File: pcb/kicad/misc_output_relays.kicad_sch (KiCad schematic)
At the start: 16 parts, among them J5 Screw_Terminal_01x03, J6 Screw_Terminal_01x03, K1 5v Relay, K2 5v Relay, Q1 MMBT3904-TP, Q2 MMBT3904-TP

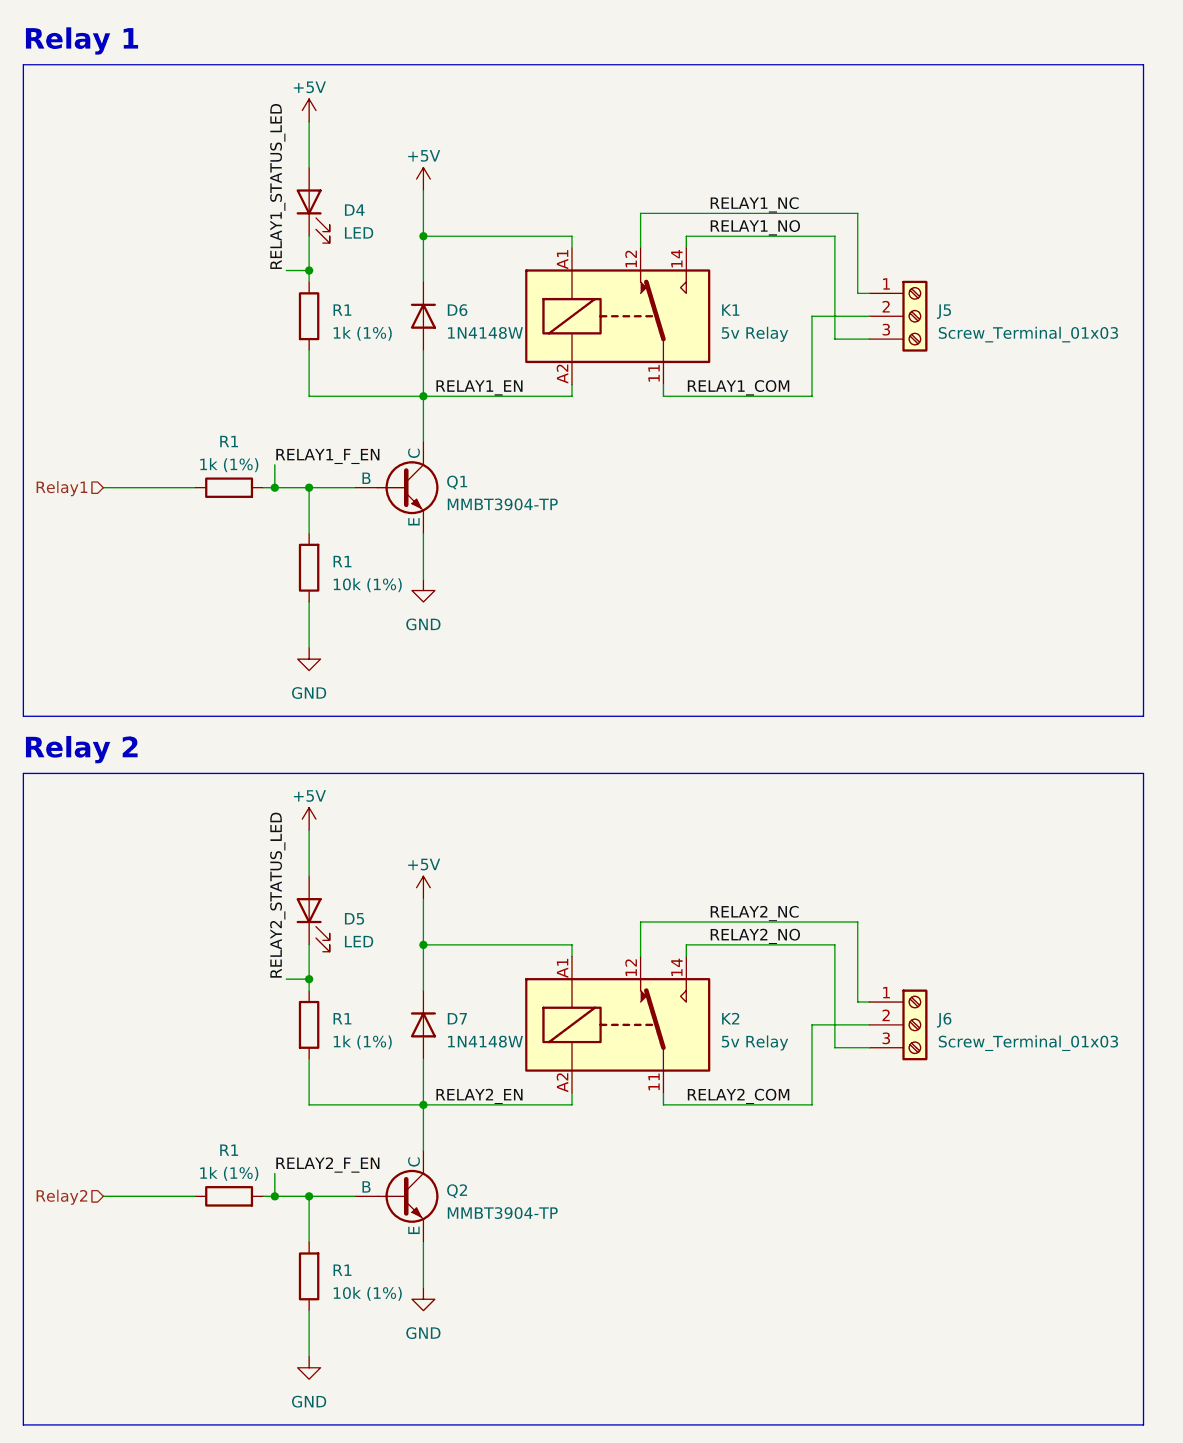
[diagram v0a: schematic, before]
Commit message: rev3-update
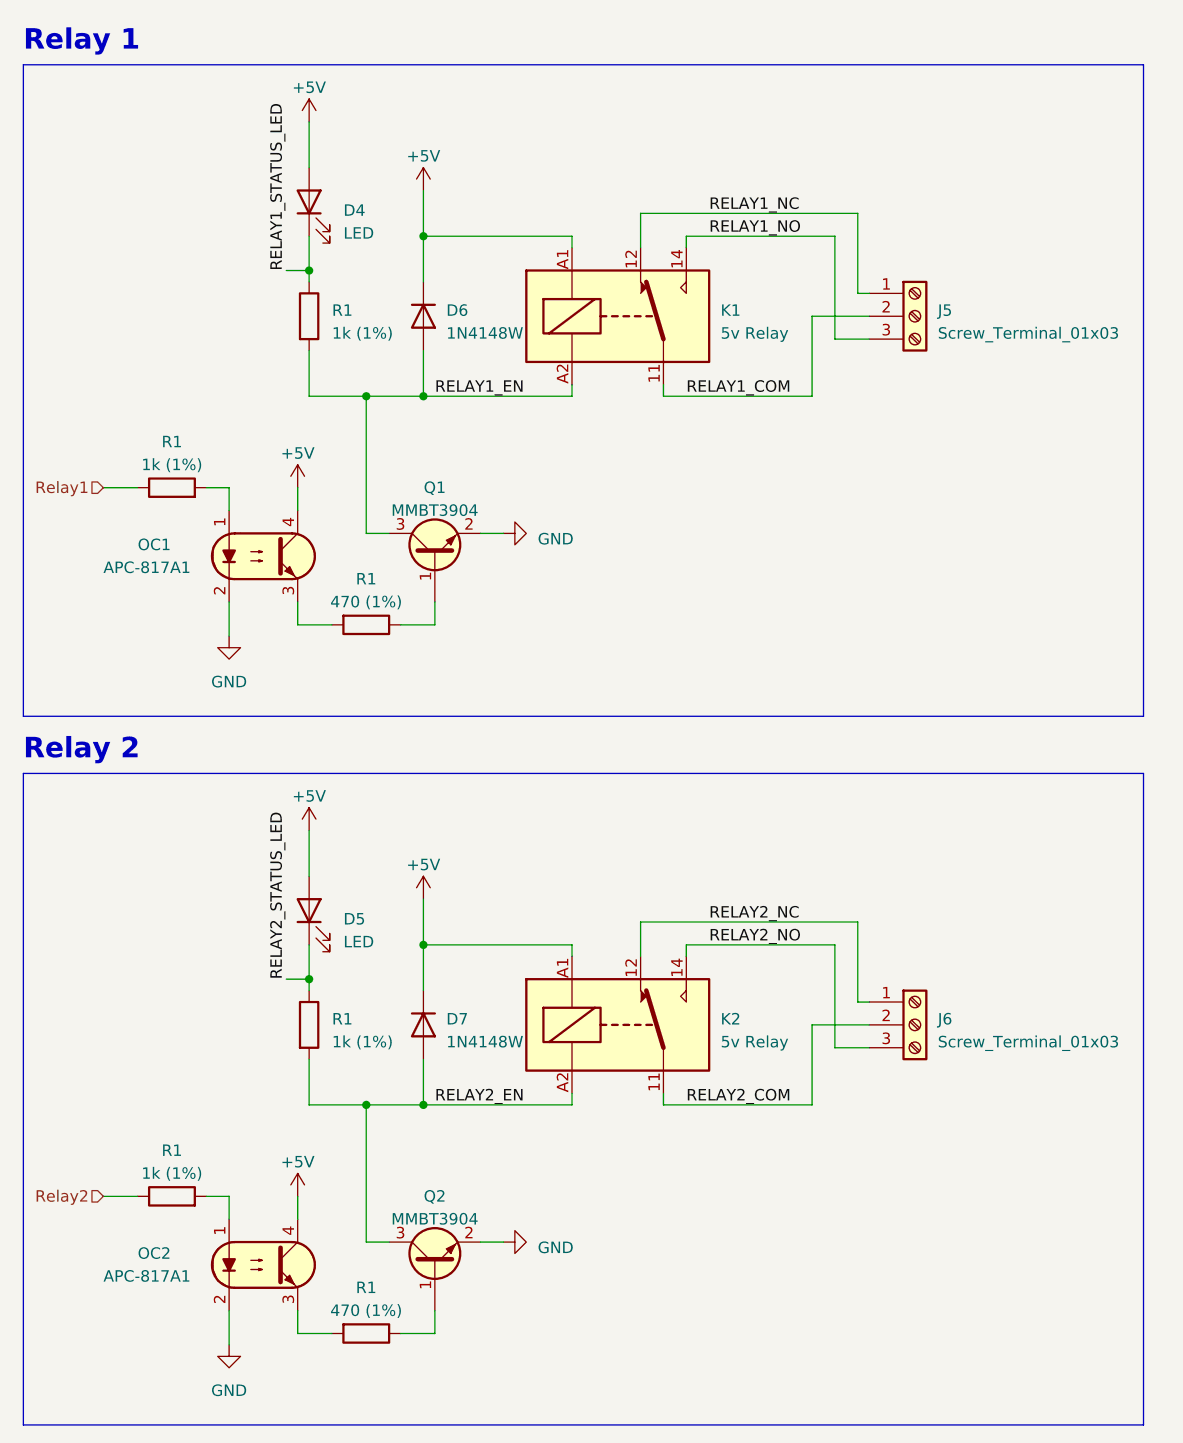
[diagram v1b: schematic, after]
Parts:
- removed Q1, Q2: MMBT3904-TP, Package_TO_SOT_SMD:SOT-23, symbol Simulation_SPICE:NPN
- removed R1: 10k (1%), PCM_Resistor_SMD_AKL:R_0603_1608Metric, symbol Device:R
- removed R1: 1k (1%), PCM_Resistor_SMD_AKL:R_0603_1608Metric, symbol Device:R
- added OC1, OC2: APC-817A1, LTV-816S:SMD4-2.54-4.6X6.5MM, symbol PCM_Optocoupler_AKL:Optocoupler_Generic
- added Q1, Q2: MMBT3904, Package_TO_SOT_SMD_AKL:SOT-23, symbol PCM_Transistor_BJT_AKL:MMBT3904
- added R1: 470 (1%), PCM_Resistor_SMD_AKL:R_0603_1608Metric, symbol Device:R
- added R1: 1k (1%), PCM_Resistor_SMD_AKL:R_0603_1608Metric, symbol Device:R
- R1: value 10k (1%) -> 470 (1%)
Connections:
- net +5V: now also OC1.4, OC2.4
- net GND: now also OC1.2, OC2.2, Q1.2 (E), Q2.2 (E); no longer R1.1
- net RELAY1_EN: now also Q1.3 (C)
- net RELAY2_EN: now also Q2.3 (C)
- net Relay2: now also R1.1
- net RELAY1_F_EN: no longer names the net of R1.2
- net RELAY1_F_EN: now also OC1.1; no longer R1.2
- new net: Q2.1 (B), R1.1
- new net: OC2.3, R1.2
- new net: Q1.1 (B), R1.1
- new net: OC1.3, R1.2
- new net: OC2.1, R1.2
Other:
- moved on the sheet: R1
